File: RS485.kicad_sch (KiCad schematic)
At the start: 8 parts, among them J7 DG390-5.0-02P, U8 XR3072XIDTR-F

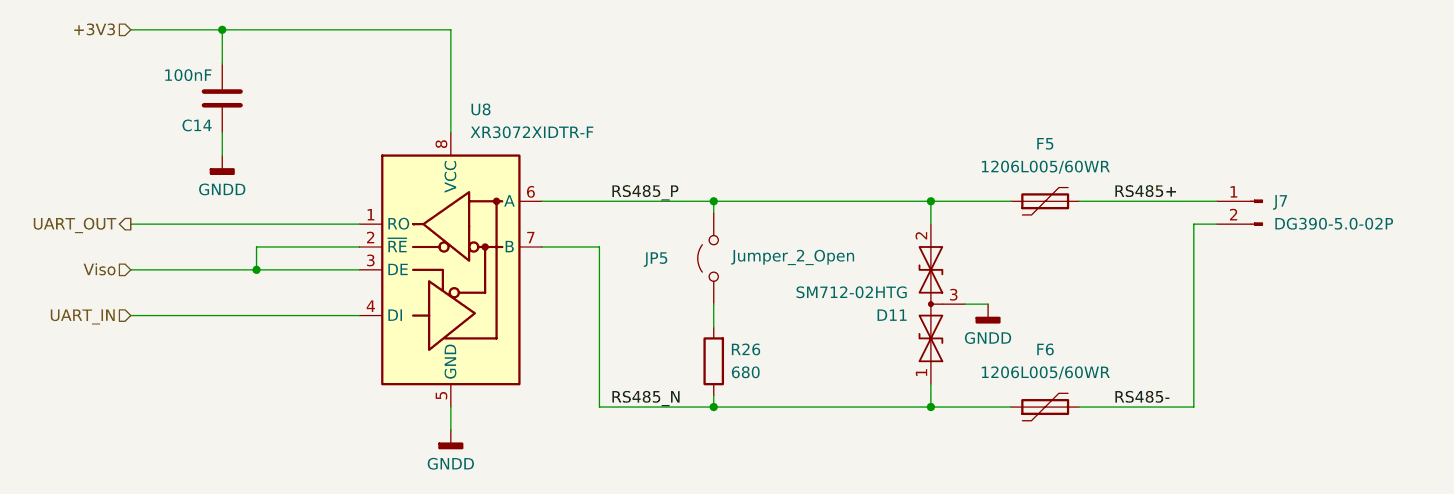
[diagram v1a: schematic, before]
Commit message: Release candidate
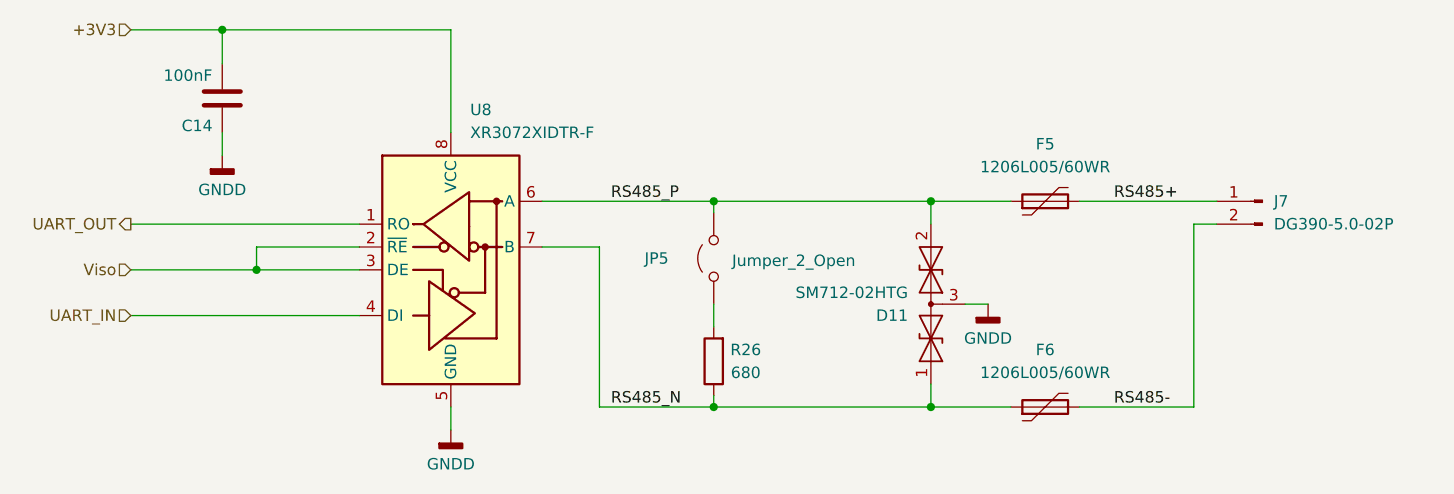
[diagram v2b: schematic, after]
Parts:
- JP5: footprint TestPoint:TestPoint_2Pads_Pitch2.54mm_Drill0.8mm -> Connector_PinHeader_2.54mm:PinHeader_1x02_P2.54mm_Vertical
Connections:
- net RS485_P: now also JP5.1 (A); no longer JP5.2 (B)
- net at R26.2: now also JP5.2 (B); no longer JP5.1 (A)
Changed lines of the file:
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@@
 (kicad_sch
-	(version 20260101)
+	(version 20260306)
 	(generator "eeschema")
 	(generator_version "10.0")
@@
 		(lib_id "Jumper:Jumper_2_Open")
 		(at 151.13 90.17 90)
+		(mirror x)
 		(unit 1)
 		(body_style 1)
@@
 		)
 		(property "Value" "Jumper_2_Open"
-			(at 160.02 89.916 90)
-			(show_name no)
-			(do_not_autoplace no)
-			(effects
-				(font
-					(size 1.27 1.27)
-				)
-			)
-		)
-		(property "Footprint" "TestPoint:TestPoint_2Pads_Pitch2.54mm_Drill0.8mm"
+			(at 160.02 90.424 90)
+			(show_name no)
+			(do_not_autoplace no)
+			(effects
+				(font
+					(size 1.27 1.27)
+				)
+			)
+		)
+		(property "Footprint" "Connector_PinHeader_2.54mm:PinHeader_1x02_P2.54mm_Vertical"
 			(at 151.13 90.17 0)
 			(hide yes)
